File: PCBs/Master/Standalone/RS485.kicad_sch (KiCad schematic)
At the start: 16 parts, among them U4 TBU-CA065-200-WH, U5 TBU-CA065-200-WH, U6 TISP4240M3BJR-S, U7 MAX487ESA+T, U8 MAX487ESA+T, U9 TISP4240M3BJR-S

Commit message: Master WIP
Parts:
- R10: footprint Resistor_SMD:R_0805_2012Metric -> Resistor_SMD:R_0402_1005Metric; LCSC C22978 -> C25890
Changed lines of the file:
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@@
     (property "Reference" "R10" (id 0) (at 173.99 128.27 90))
     (property "Value" "3.3K" (id 1) (at 173.99 130.81 90))
-    (property "Footprint" "Resistor_SMD:R_0805_2012Metric" (id 2) (at 173.99 132.842 90)
+    (property "Footprint" "Resistor_SMD:R_0402_1005Metric" (id 2) (at 173.99 132.842 90)
       (effects (font (size 1.27 1.27)) hide)
     )
@@
       (effects (font (size 1.27 1.27)) hide)
     )
-    (property "LCSC" "C22978" (id 4) (at 173.99 134.62 0)
+    (property "LCSC" "C25890" (id 4) (at 173.99 134.62 0)
       (effects (font (size 1.27 1.27)) hide)
     )

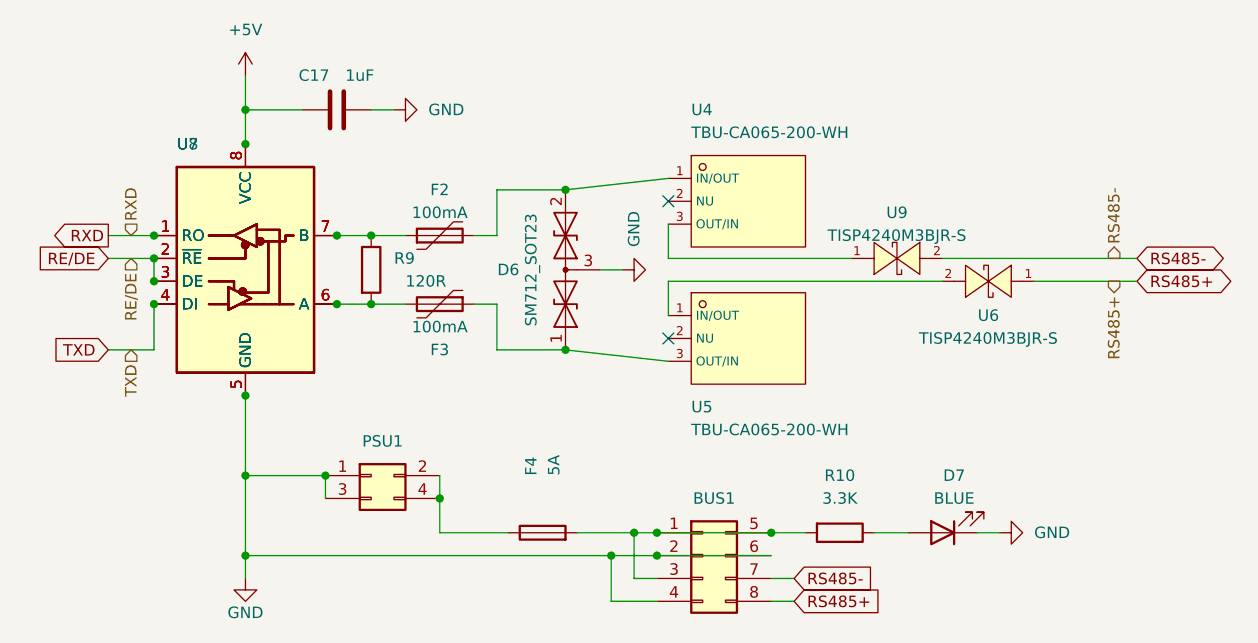
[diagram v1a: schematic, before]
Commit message: Master Rev. 1
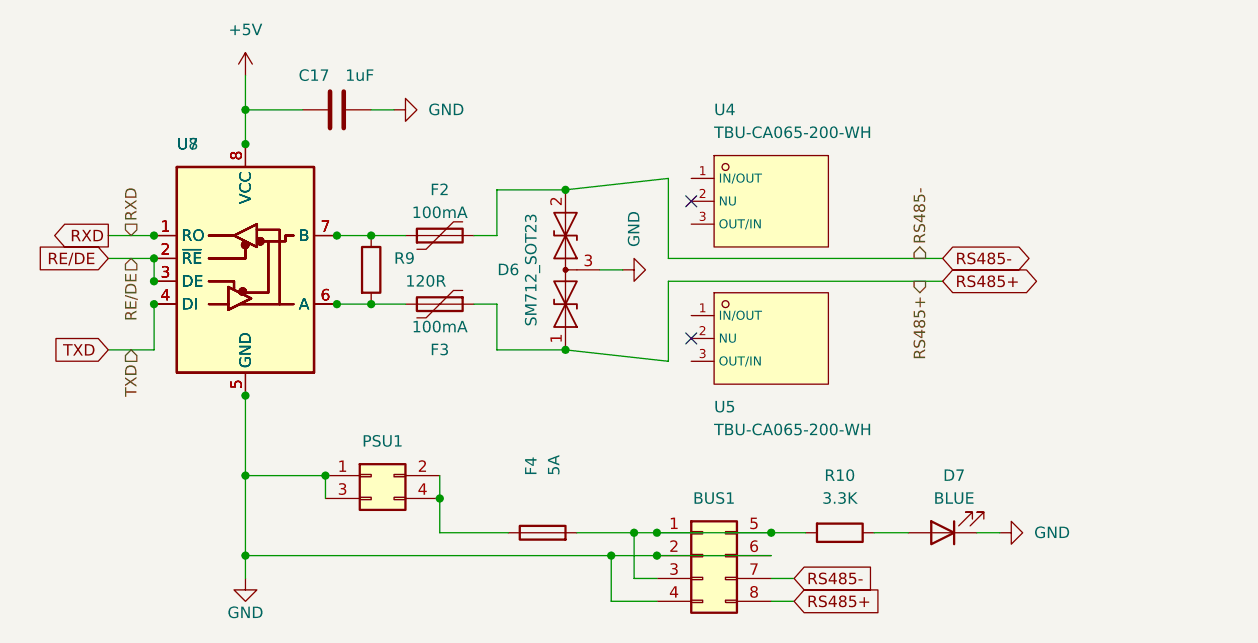
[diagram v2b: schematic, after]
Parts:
- removed U6, U9: TISP4240M3BJR-S, A10 KiCad Libraries:DO-214AA_L4.4-W3.6-LS5.3-BI, symbol A10:TISP4240M3BJR-S
- F4: footprint A10 KiCad Libraries:FUSE_BK-6013 -> A10 KiCad Libraries:FUSE-TH_XF-506P
- U4, U5: now left out of the parts list
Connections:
- net RS485+: now also D6.1 (A1), F3.1
- net RS485-: now also D6.2 (A2), F2.2
- now unconnected: U4.1 (IN/OUT), U5.3 (OUT/IN)
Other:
- moved on the sheet: U4, U5
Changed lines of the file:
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@@
   (junction (at 97.79 106.68) (diameter 0) (color 0 0 0 0)
   )
-  (no_connect (at 154.94 97.79))
-  (no_connect (at 154.94 113.03))
+  (no_connect (at 157.48 97.79))
+  (no_connect (at 157.48 113.03))
   (wire (pts (xy 143.51 96.52) (xy 154.94 95.25))
     (stroke (width 0) (type default) (color 0 0 0 0))
@@
     (stroke (width 0) (type default) (color 0 0 0 0))
   )
-  (wire (pts (xy 185.42 106.68) (xy 154.94 106.68))
-    (stroke (width 0) (type default) (color 0 0 0 0))
-  )
   (wire (pts (xy 116.84 128.27) (xy 116.84 130.81))
     (stroke (width 0) (type default) (color 0 0 0 0))
   )
-  (wire (pts (xy 154.94 106.68) (xy 154.94 110.49))
-    (stroke (width 0) (type default) (color 0 0 0 0))
-  )
   (wire (pts (xy 166.37 134.62) (xy 170.18 134.62))
     (stroke (width 0) (type default) (color 0 0 0 0))
@@
     (stroke (width 0) (type default) (color 0 0 0 0))
   )
-  (wire (pts (xy 185.42 104.14) (xy 207.01 104.14))
+  (wire (pts (xy 154.94 104.14) (xy 185.42 104.14))
     (stroke (width 0) (type default) (color 0 0 0 0))
   )
@@
     (stroke (width 0) (type default) (color 0 0 0 0))
   )
-  (wire (pts (xy 195.58 106.68) (xy 207.01 106.68))
-    (stroke (width 0) (type default) (color 0 0 0 0))
-  )
-  (wire (pts (xy 154.94 100.33) (xy 154.94 104.14))
+  (wire (pts (xy 154.94 106.68) (xy 185.42 106.68))
+    (stroke (width 0) (type default) (color 0 0 0 0))
+  )
+  (wire (pts (xy 154.94 95.25) (xy 154.94 104.14))
     (stroke (width 0) (type default) (color 0 0 0 0))
   )
@@
     (stroke (width 0) (type default) (color 0 0 0 0))
   )
+  (wire (pts (xy 154.94 106.68) (xy 154.94 115.57))
+    (stroke (width 0) (type default) (color 0 0 0 0))
+  )
   (wire (pts (xy 107.95 83.82) (xy 107.95 87.63))
     (stroke (width 0) (type default) (color 0 0 0 0))
@@
   )
   (wire (pts (xy 168.91 139.7) (xy 166.37 139.7))
-    (stroke (width 0) (type default) (color 0 0 0 0))
-  )
-  (wire (pts (xy 154.94 104.14) (xy 175.26 104.14))
     (stroke (width 0) (type default) (color 0 0 0 0))
   )
@@
     )
   )
-  (global_label "RS485+" (shape bidirectional) (at 207.01 106.68 0) (fields_autoplaced)
+  (global_label "RS485+" (shape bidirectional) (at 185.42 106.68 0) (fields_autoplaced)
     (effects (font (size 1.27 1.27)) (justify left))
-    (property "Intersheet References" "${INTERSHEET_REFS}" (id 0) (at 217.1036 106.7594 0)
+    (property "Intersheet References" "${INTERSHEET_REFS}" (id 0) (at 195.5136 106.7594 0)
       (effects (font (size 1.27 1.27)) (justify left) hide)
     )
@@
     )
   )
-  (global_label "RS485-" (shape bidirectional) (at 207.01 104.14 0) (fields_autoplaced)
+  (global_label "RS485-" (shape bidirectional) (at 185.42 104.14 0) (fields_autoplaced)
     (effects (font (size 1.27 1.27)) (justify left))
-    (property "Intersheet References" "${INTERSHEET_REFS}" (id 0) (at 217.1036 104.2194 0)
+    (property "Intersheet References" "${INTERSHEET_REFS}" (id 0) (at 195.5136 104.2194 0)
       (effects (font (size 1.27 1.27)) (justify left) hide)
     )
@@
     (effects (font (size 1.27 1.27)) (justify right))
   )
-  (hierarchical_label "RS485-" (shape output) (at 204.47 104.14 90)
+  (hierarchical_label "RS485-" (shape output) (at 182.88 104.14 90)
     (effects (font (size 1.27 1.27)) (justify left))
   )
-  (hierarchical_label "RS485+" (shape output) (at 204.47 106.68 270)
+  (hierarchical_label "RS485+" (shape output) (at 182.88 106.68 270)
     (effects (font (size 1.27 1.27)) (justify right))
   )
@@
     (pin "2")
     (pin "3")
-  )
-  (symbol (lib_id "A10:TISP4240M3BJR-S") (at 187.96 99.06 0) (unit 1)
-    (in_bom yes) (on_board yes)
-    (property "Reference" "U6" (id 0) (at 190.5 110.49 0))
-    (property "Value" "TISP4240M3BJR-S" (id 1) (at 190.5 113.03 0))
-    (property "Footprint" "A10 KiCad Libraries:DO-214AA_L4.4-W3.6-LS5.3-BI" (id 2) (at 187.96 109.22 0)
-      (effects (font (size 1.27 1.27) italic) hide)
-    )
-    (property "Datasheet" "https://atta.szlcsc.com/upload/public/pdf/source/20210316/C2760879_B8B4F1F8D05F3CAAD32384151EC07A7F.pdf" (id 3) (at 185.674 98.933 0)
-      (effects (font (size 1.27 1.27)) (justify left) hide)
-    )
-    (property "LCSC" "C840526" (id 4) (at 187.96 99.06 0)
-      (effects (font (size 1.27 1.27)) hide)
-    )
-    (pin "1")
-    (pin "2")
   )
   (symbol (lib_id "Connector_Generic:Conn_02x02_Odd_Even") (at 121.92 128.27 0) (unit 1)
@@
     (pin "4")
   )
-  (symbol (lib_name "TBU-CA065-200-WH_1") (lib_id "A10:TBU-CA065-200-WH") (at 154.94 74.93 0) (unit 1)
-    (in_bom yes) (on_board yes)
-    (property "Reference" "U4" (id 0) (at 157.48 87.63 0)
-      (effects (font (size 1.27 1.27)) (justify left))
-    )
-    (property "Value" "TBU-CA065-200-WH" (id 1) (at 157.48 90.17 0)
-      (effects (font (size 1.27 1.27)) (justify left))
-    )
-    (property "Footprint" "A10 KiCad Libraries:DIO-SMD_3P-L6.5-W4.0-BI" (id 2) (at 154.94 85.09 0)
+  (symbol (lib_name "TBU-CA065-200-WH_1") (lib_id "A10:TBU-CA065-200-WH") (at 157.48 74.93 0) (unit 1)
+    (in_bom no) (on_board no)
+    (property "Reference" "U4" (id 0) (at 160.02 87.63 0)
+      (effects (font (size 1.27 1.27)) (justify left))
+    )
+    (property "Value" "TBU-CA065-200-WH" (id 1) (at 160.02 90.17 0)
+      (effects (font (size 1.27 1.27)) (justify left))
+    )
+    (property "Footprint" "A10 KiCad Libraries:DIO-SMD_3P-L6.5-W4.0-BI" (id 2) (at 157.48 85.09 0)
       (effects (font (size 1.27 1.27) italic) hide)
     )
-    (property "Datasheet" "https://atta.szlcsc.com/upload/public/pdf/source/20200810/C720638_9C2F93931169B2F615A5326102BC91F1.pdf" (id 3) (at 152.654 74.803 0)
-      (effects (font (size 1.27 1.27)) (justify left) hide)
-    )
-    (property "LCSC" "C913221" (id 4) (at 154.94 74.93 0)
+    (property "Datasheet" "https://atta.szlcsc.com/upload/public/pdf/source/20200810/C720638_9C2F93931169B2F615A5326102BC91F1.pdf" (id 3) (at 155.194 74.803 0)
+      (effects (font (size 1.27 1.27)) (justify left) hide)
+    )
+    (property "LCSC" "C913221" (id 4) (at 157.48 74.93 0)
       (effects (font (size 1.27 1.27)) hide)
     )
@@
     (pin "8")
   )
-  (symbol (lib_id "A10:TISP4240M3BJR-S") (at 182.88 111.76 180) (unit 1)
-    (in_bom yes) (on_board yes) (fields_autoplaced)
-    (property "Reference" "U9" (id 0) (at 180.34 99.06 0))
-    (property "Value" "TISP4240M3BJR-S" (id 1) (at 180.34 101.6 0))
-    (property "Footprint" "A10 KiCad Libraries:DO-214AA_L4.4-W3.6-LS5.3-BI" (id 2) (at 182.88 101.6 0)
-      (effects (font (size 1.27 1.27) italic) hide)
-    )
-    (property "Datasheet" "https://atta.szlcsc.com/upload/public/pdf/source/20210316/C2760879_B8B4F1F8D05F3CAAD32384151EC07A7F.pdf" (id 3) (at 185.166 111.887 0)
-      (effects (font (size 1.27 1.27)) (justify left) hide)
-    )
-    (property "LCSC" "C840526" (id 4) (at 182.88 111.76 0)
-      (effects (font (size 1.27 1.27)) hide)
-    )
-    (pin "1")
-    (pin "2")
-  )
   (symbol (lib_id "power:GND") (at 124.46 87.63 90) (unit 1)
     (in_bom yes) (on_board yes) (fields_autoplaced)
@@
       (effects (font (size 1.27 1.27)) (justify left))
     )
-    (property "Footprint" "A10 KiCad Libraries:FUSE_BK-6013" (id 2) (at 140.97 136.398 90)
+    (property "Footprint" "A10 KiCad Libraries:FUSE-TH_XF-506P" (id 2) (at 140.97 136.398 90)
       (effects (font (size 1.27 1.27)) hide)
     )
@@
     (pin "8")
   )
-  (symbol (lib_name "TBU-CA065-200-WH_1") (lib_id "A10:TBU-CA065-200-WH") (at 154.94 90.17 0) (unit 1)
-    (in_bom yes) (on_board yes)
-    (property "Reference" "U5" (id 0) (at 157.48 120.65 0)
-      (effects (font (size 1.27 1.27)) (justify left))
-    )
-    (property "Value" "TBU-CA065-200-WH" (id 1) (at 157.48 123.19 0)
-      (effects (font (size 1.27 1.27)) (justify left))
-    )
-    (property "Footprint" "A10 KiCad Libraries:DIO-SMD_3P-L6.5-W4.0-BI" (id 2) (at 154.94 100.33 0)
+  (symbol (lib_name "TBU-CA065-200-WH_1") (lib_id "A10:TBU-CA065-200-WH") (at 157.48 90.17 0) (unit 1)
+    (in_bom no) (on_board no)
+    (property "Reference" "U5" (id 0) (at 160.02 120.65 0)
+      (effects (font (size 1.27 1.27)) (justify left))
+    )
+    (property "Value" "TBU-CA065-200-WH" (id 1) (at 160.02 123.19 0)
+      (effects (font (size 1.27 1.27)) (justify left))
+    )
+    (property "Footprint" "A10 KiCad Libraries:DIO-SMD_3P-L6.5-W4.0-BI" (id 2) (at 157.48 100.33 0)
       (effects (font (size 1.27 1.27) italic) hide)
     )
-    (property "Datasheet" "https://atta.szlcsc.com/upload/public/pdf/source/20200810/C720638_9C2F93931169B2F615A5326102BC91F1.pdf" (id 3) (at 152.654 90.043 0)
-      (effects (font (size 1.27 1.27)) (justify left) hide)
-    )
-    (property "LCSC" "C913221" (id 4) (at 154.94 90.17 0)
-      (effects (font (size 1.27 1.27)) hide)
-    )
+    (property "Datasheet" "https://atta.szlcsc.com/upload/public/pdf/source/20200810/C720638_9C2F93931169B2F615A5326102BC91F1.pdf" (id 3) (at 155.194 90.043 0)
+      (effects (font (size 1.27 1.27)) (justify left) hide)
+    )
+    (property "LCSC" "C913221" (id 4) (at 157.48 90.17 0)
+      (effects (font (size 1.27 1.27)) hide)
+    )
